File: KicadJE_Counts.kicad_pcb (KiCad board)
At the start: 2 copper layers, 242 x 128 mm, 215 parts, among them J108 Conn_02x03_Male, J201 ClockOut, J202 ClockIn, J203 Out0, J204 Out1, J205 Out2, J206 Out3, J207 Out4, J208 Out5, J209 Out6, J210 Out7, J211 Out8, J212 Out9, J213 Reset, J214 Hold, J301 Doepfer connector, J302 In_1, J303 In 2, J304 Out 1, J305 Out 2, J306 Out 1 Final, J307 Out 2 Final, P201 HEADER_2x5_Doepfer, SW201 Run, U201 LM555, U202 4017, U301 TL072, U302 TL072

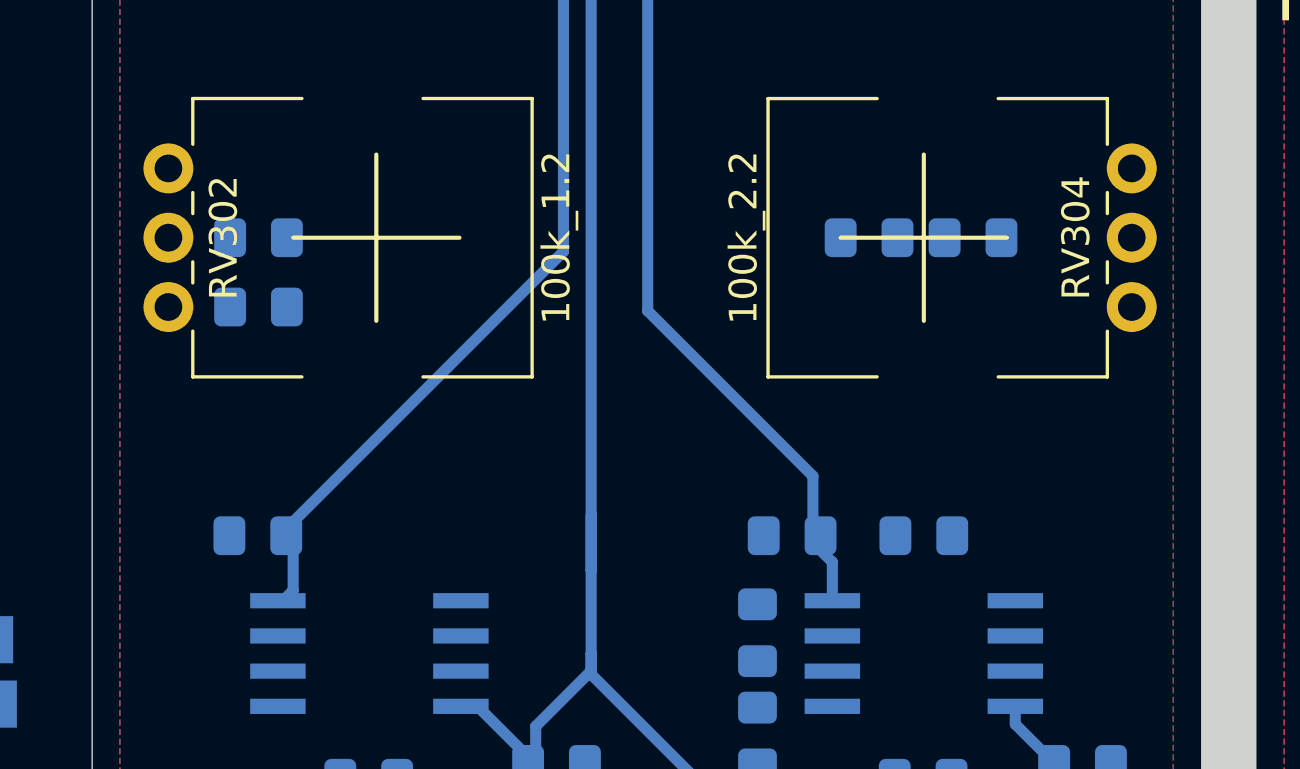
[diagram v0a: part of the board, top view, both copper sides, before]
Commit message: Update KicadJE_Counts.kicad_pcb
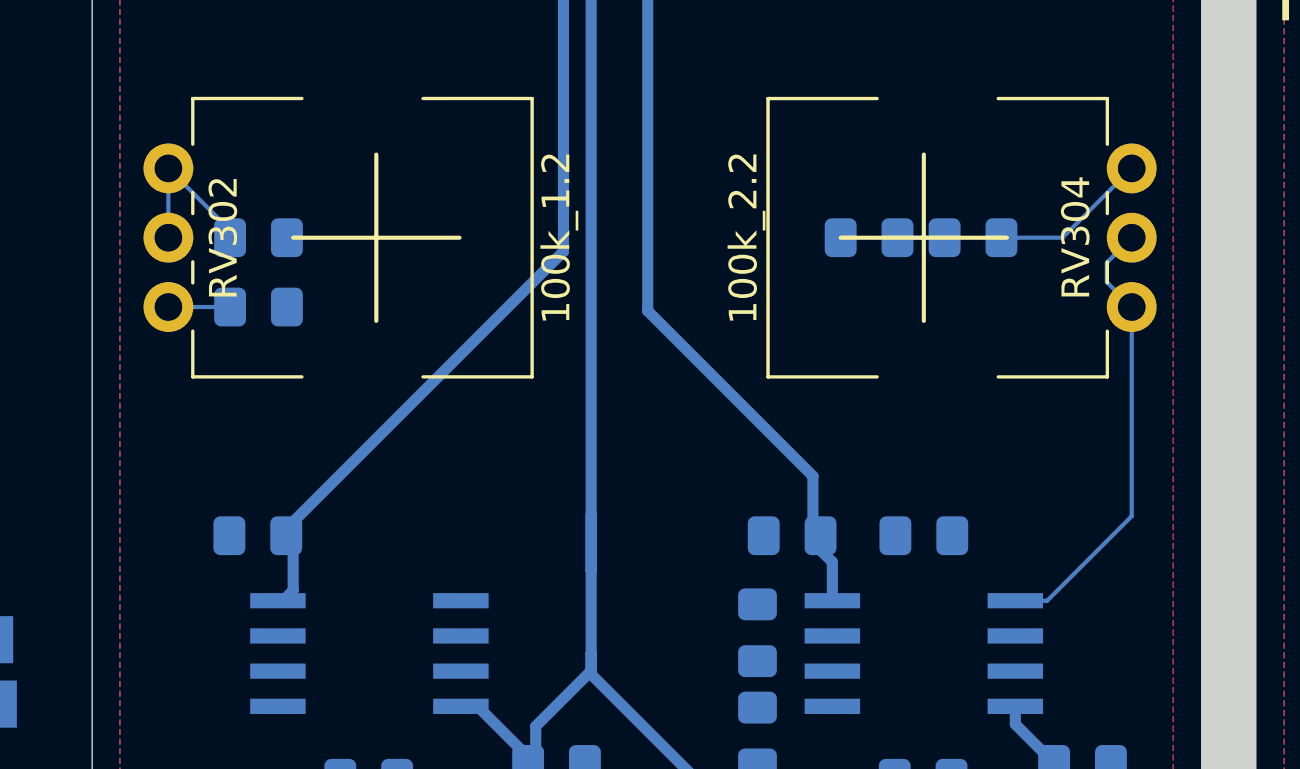
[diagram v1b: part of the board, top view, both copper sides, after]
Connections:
- net /KicadJE_Counts2/POT2_L renamed POT2_L
- net /KicadJE_Counts2/POT3_L renamed POT3_L
- net /KicadJE_Counts2/POT4_L renamed POT4_L
- R314 pad 1: /KicadJE_Counts2/POT3_C -> POT3_C
- R317 pad 1: /KicadJE_Counts2/POT3_C -> POT3_C
- R322 pad 2: /KicadJE_Counts2/POT3_C -> POT3_C
- R327 pad 2: /KicadJE_Counts2/POT4_C -> POT4_C
- R328 pad 1: /KicadJE_Counts2/POT2_C -> POT2_C
- R330 pad 2: /KicadJE_Counts2/POT4_C -> POT4_C
- RV302 pad 2: /KicadJE_Counts2/POT2_C -> POT2_C
- RV302 pad 3: (no net) -> POT2_C
- RV303 pad 2: /KicadJE_Counts2/POT3_C -> POT3_C
- RV303 pad 3: (no net) -> POT3_C
- RV304 pad 2: /KicadJE_Counts2/POT4_C -> POT4_C
- RV304 pad 3: (no net) -> POT4_C
- U301 pad 1: /KicadJE_Counts2/POT4_C -> POT4_C
- U301 pad 7: /KicadJE_Counts2/POT3_C -> POT3_C
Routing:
- net POT4_C: track 0.00 -> 16.3 mm
- net POT2_C: track 0.00 -> 5.92 mm
- net POT4_L: track 0.00 -> 5.74 mm
- net POT2_L: track 0.00 -> 2.23 mm
- net Net-(R320-Pad1): track 0.00 -> 1.70 mm
